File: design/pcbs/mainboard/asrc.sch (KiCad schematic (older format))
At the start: 18 parts, among them J9 Conn_01x03, U10 TPS79318-EP, U11 SRC4392

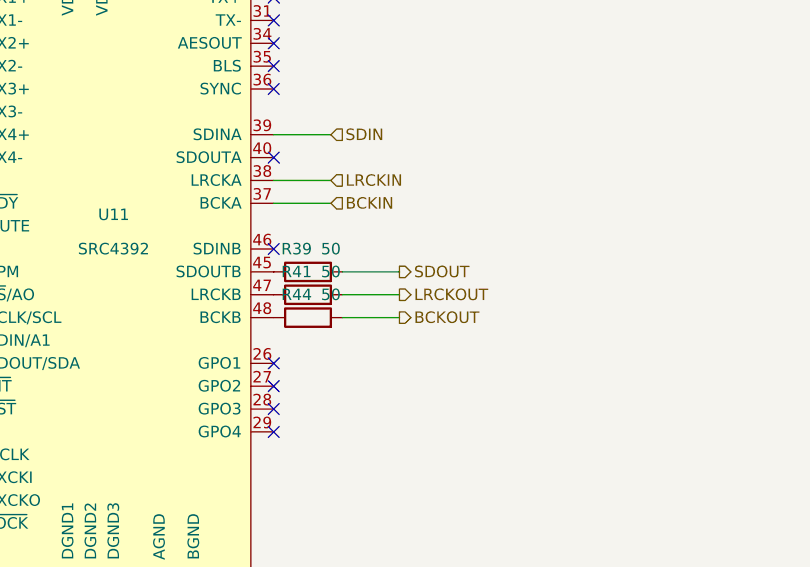
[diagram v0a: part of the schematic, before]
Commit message: Misc updates
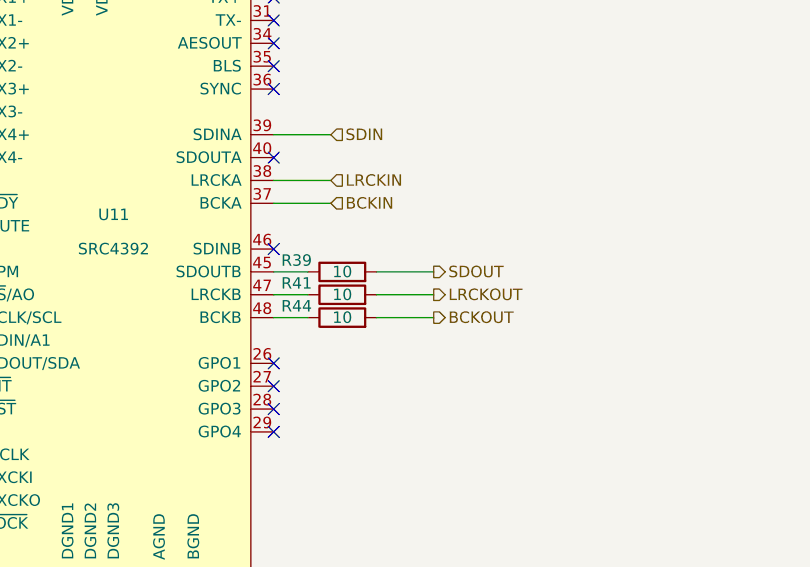
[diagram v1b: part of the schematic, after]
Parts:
- R39, R41, R44: value 50 -> 10; LCSC C25082 -> C25077
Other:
- moved on the sheet: R39, R41, R44
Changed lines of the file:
@@
 $EndComp
 Wire Wire Line
-	5950 5050 5700 5050
+	6100 5050 5850 5050
 Wire Wire Line
-	5700 4950 5950 4950
-Text HLabel 5950 5050 2    50   Output ~ 0
+	5850 4950 6100 4950
+Text HLabel 6100 5050 2    50   Output ~ 0
 BCKOUT
-Text HLabel 5950 4950 2    50   Output ~ 0
+Text HLabel 6100 4950 2    50   Output ~ 0
 LRCKOUT
 Wire Wire Line
-	5700 4850 5950 4850
-Text HLabel 5950 4850 2    50   Output ~ 0
+	5850 4850 6100 4850
+Text HLabel 6100 4850 2    50   Output ~ 0
 SDOUT
 $Comp
 L Device:R R?
 U 1 1 5EEA869D
-P 5550 4850
+P 5700 4850
 AR Path="/5EEA869D" Ref="R?"  Part="1"
 AR Path="/5EC77FFA/5EEA869D" Ref="R39"  Part="1"
-F 0 "R39" V 5650 4900 50  0000 C CNN
-F 1 "50" V 5650 4750 50  0000 C CNN
-F 2 "Resistor_SMD:R_0402_1005Metric" V 5480 4850 50  0001 C CNN
-F 3 "https://datasheet.lcsc.com/szlcsc/Uniroyal-Elec-0402WGF1500TCE_C25082.pdf" H 5550 4850 50  0001 C CNN
-F 4 "C25082" H 5550 4850 50  0001 C CNN "LCSC"
-F 5 "Yes" H 5550 4850 50  0001 C CNN "Done"
-F 6 "Termination" H 5550 4850 50  0001 C CNN "Function"
-	1    5550 4850
+F 0 "R39" V 5750 5050 50  0000 C CNN
+F 1 "10" V 5700 4850 50  0000 C CNN
+F 2 "Resistor_SMD:R_0402_1005Metric" V 5630 4850 50  0001 C CNN
+F 3 "Uniroyal-Elec-0402WGF100JTCE_C25077.pdf" H 5700 4850 50  0001 C CNN
+F 4 "C25077" H 5700 4850 50  0001 C CNN "LCSC"
+F 5 "Yes" H 5700 4850 50  0001 C CNN "Done"
+F 6 "Termination" H 5700 4850 50  0001 C CNN "Function"
+	1    5700 4850
 	0    -1   -1   0
 $EndComp
@@
 L Device:R R?
 U 1 1 5EEAFFEA
-P 5550 4950
+P 5700 4950
 AR Path="/5EEAFFEA" Ref="R?"  Part="1"
 AR Path="/5EC77FFA/5EEAFFEA" Ref="R41"  Part="1"
-F 0 "R41" V 5650 5000 50  0000 C CNN
-F 1 "50" V 5650 4850 50  0000 C CNN
-F 2 "Resistor_SMD:R_0402_1005Metric" V 5480 4950 50  0001 C CNN
-F 3 "https://datasheet.lcsc.com/szlcsc/Uniroyal-Elec-0402WGF1500TCE_C25082.pdf" H 5550 4950 50  0001 C CNN
-F 4 "C25082" H 5550 4950 50  0001 C CNN "LCSC"
-F 5 "Yes" H 5550 4950 50  0001 C CNN "Done"
-F 6 "Termination" H 5550 4950 50  0001 C CNN "Function"
-	1    5550 4950
+F 0 "R41" V 5750 5150 50  0000 C CNN
+F 1 "10" V 5700 4950 50  0000 C CNN
+F 2 "Resistor_SMD:R_0402_1005Metric" V 5630 4950 50  0001 C CNN
+F 3 "Uniroyal-Elec-0402WGF100JTCE_C25077.pdf" H 5700 4950 50  0001 C CNN
+F 4 "C25077" H 5700 4950 50  0001 C CNN "LCSC"
+F 5 "Yes" H 5700 4950 50  0001 C CNN "Done"
+F 6 "Termination" H 5700 4950 50  0001 C CNN "Function"
+	1    5700 4950
 	0    -1   -1   0
 $EndComp
@@
 L Device:R R?
 U 1 1 5EEB02AB
-P 5550 5050
+P 5700 5050
 AR Path="/5EEB02AB" Ref="R?"  Part="1"
 AR Path="/5EC77FFA/5EEB02AB" Ref="R44"  Part="1"
-F 0 "R44" V 5650 5100 50  0000 C CNN
-F 1 "50" V 5650 4950 50  0000 C CNN
-F 2 "Resistor_SMD:R_0402_1005Metric" V 5480 5050 50  0001 C CNN
-F 3 "https://datasheet.lcsc.com/szlcsc/Uniroyal-Elec-0402WGF1500TCE_C25082.pdf" H 5550 5050 50  0001 C CNN
-F 4 "C25082" H 5550 5050 50  0001 C CNN "LCSC"
-F 5 "Yes" H 5550 5050 50  0001 C CNN "Done"
-F 6 "Termination" H 5550 5050 50  0001 C CNN "Function"
-	1    5550 5050
+F 0 "R44" V 5750 5250 50  0000 C CNN
+F 1 "10" V 5700 5050 50  0000 C CNN
+F 2 "Resistor_SMD:R_0402_1005Metric" V 5630 5050 50  0001 C CNN
+F 3 "Uniroyal-Elec-0402WGF100JTCE_C25077.pdf" H 5700 5050 50  0001 C CNN
+F 4 "C25077" H 5700 5050 50  0001 C CNN "LCSC"
+F 5 "Yes" H 5700 5050 50  0001 C CNN "Done"
+F 6 "Termination" H 5700 5050 50  0001 C CNN "Function"
+	1    5700 5050
 	0    -1   -1   0
 $EndComp
+Wire Wire Line
+	5550 4850 5400 4850
+Wire Wire Line
+	5400 5050 5550 5050
+Wire Wire Line
+	5550 4950 5400 4950
 $EndSCHEMATC
